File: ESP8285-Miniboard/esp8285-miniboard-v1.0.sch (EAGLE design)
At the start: 40 parts, among them Q1 FA-128

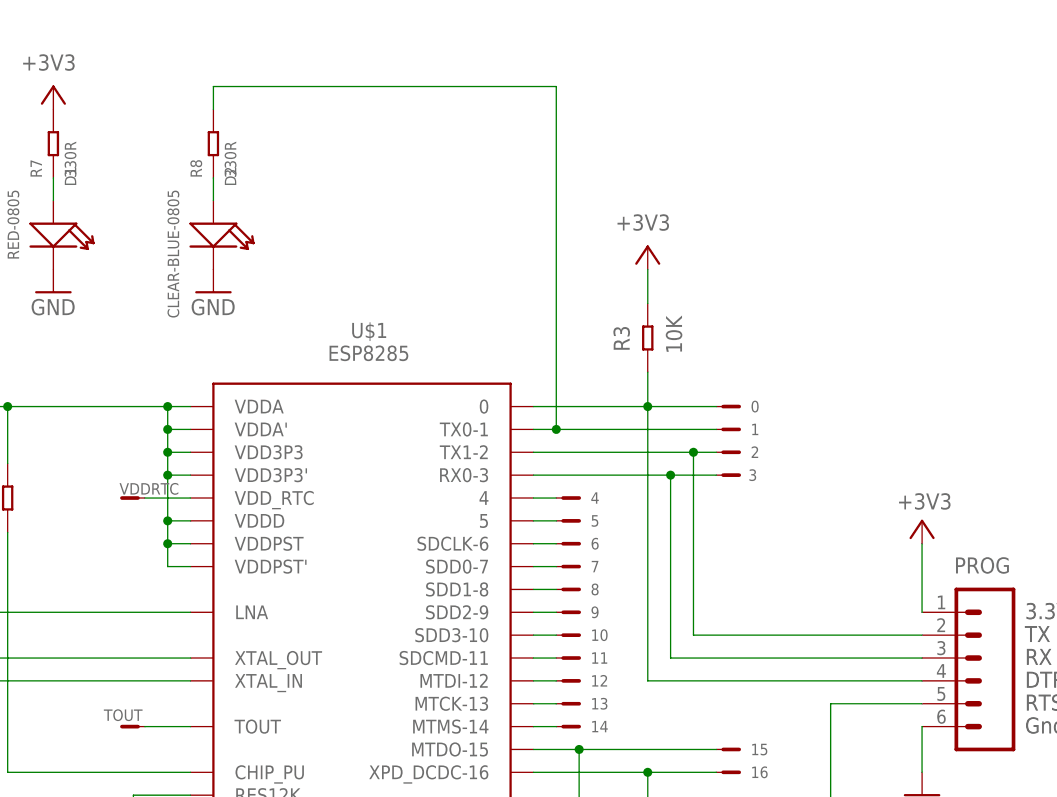
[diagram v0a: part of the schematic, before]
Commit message: Another Rev 1.0
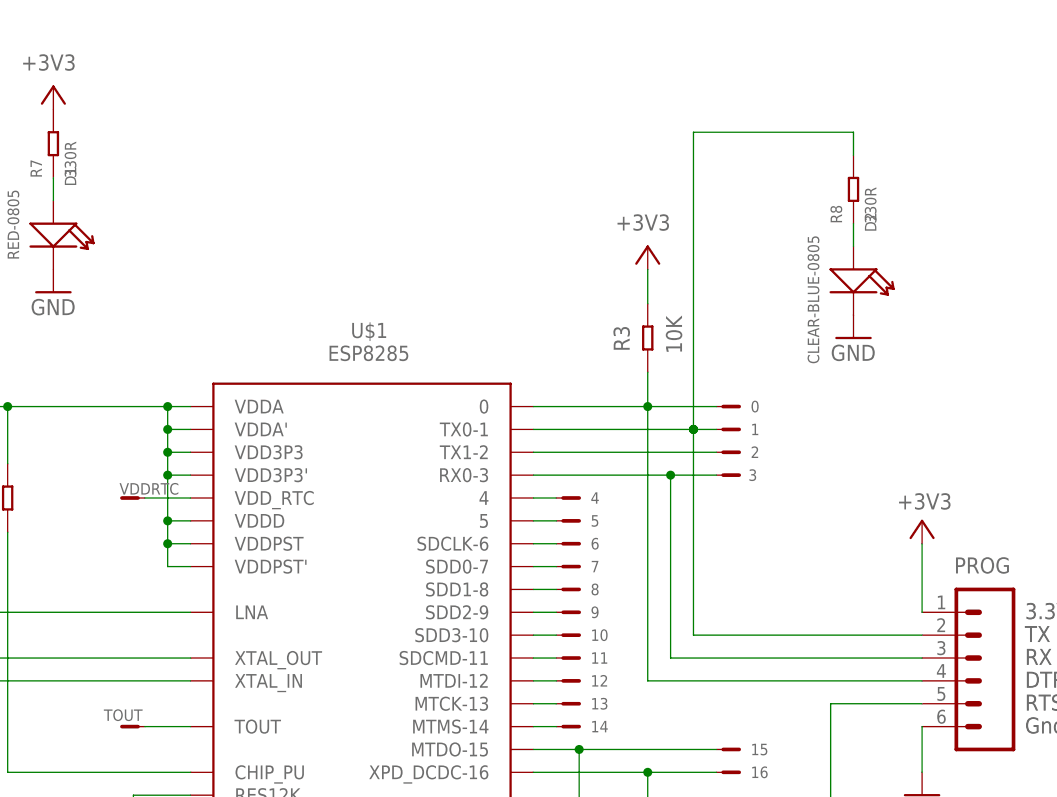
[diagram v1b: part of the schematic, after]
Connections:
- net N$IO1: now also PROG.2
- net N$IO2: no longer PROG.2
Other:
- moved on the sheet: D2, R8
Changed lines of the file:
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@@
 <attribute name="VALUE" x="91.44" y="163.576" size="1.778" layer="96" rot="R180"/>
 </instance>
-<instance part="D2" gate="G$1" x="106.68" y="143.51" rot="R270"/>
-<instance part="R8" gate="G$1" x="106.68" y="153.67" rot="R90"/>
-<instance part="GND13" gate="1" x="106.68" y="137.16"/>
+<instance part="D2" gate="G$1" x="177.8" y="138.43" rot="R270"/>
+<instance part="R8" gate="G$1" x="177.8" y="148.59" rot="R90"/>
+<instance part="GND13" gate="1" x="177.8" y="132.08"/>
 </instances>
 <busses>
@@
 </segment>
 </net>
-<net name="N$IO2" class="0">
-<segment>
-<wire x1="160.02" y1="99.06" x2="185.42" y2="99.06" width="0.1524" layer="91"/>
-<pinref part="PROG" gate="G$1" pin="2"/>
-<pinref part="U$1" gate="G$1" pin="TX1-2"/>
-<pinref part="2" gate="G$1" pin="1"/>
-<wire x1="162.56" y1="119.38" x2="160.02" y2="119.38" width="0.1524" layer="91"/>
-<wire x1="160.02" y1="119.38" x2="142.24" y2="119.38" width="0.1524" layer="91"/>
-<wire x1="160.02" y1="99.06" x2="160.02" y2="119.38" width="0.1524" layer="91"/>
-<junction x="160.02" y="119.38"/>
-</segment>
-</net>
 <net name="N$IO3" class="0">
 <segment>
@@
 <pinref part="D2" gate="G$1" pin="+"/>
 <pinref part="R8" gate="G$1" pin="1"/>
-<wire x1="106.68" y1="149.86" x2="106.68" y2="147.32" width="0.1524" layer="91"/>
+<wire x1="177.8" y1="144.78" x2="177.8" y2="142.24" width="0.1524" layer="91"/>
+</segment>
+</net>
+<net name="N$IO2" class="0">
+<segment>
+<pinref part="U$1" gate="G$1" pin="TX1-2"/>
+<pinref part="2" gate="G$1" pin="1"/>
+<wire x1="162.56" y1="119.38" x2="142.24" y2="119.38" width="0.1524" layer="91"/>
 </segment>
 </net>
 <net name="N$IO1" class="0">
 <segment>
-<wire x1="106.68" y1="160.02" x2="106.68" y2="157.48" width="0.1524" layer="91"/>
+<wire x1="160.02" y1="99.06" x2="185.42" y2="99.06" width="0.1524" layer="91"/>
+<pinref part="PROG" gate="G$1" pin="2"/>
+<wire x1="177.8" y1="154.94" x2="177.8" y2="152.4" width="0.1524" layer="91"/>
 <pinref part="R8" gate="G$1" pin="2"/>
 <pinref part="1" gate="G$1" pin="1"/>
 <pinref part="U$1" gate="G$1" pin="TX0-1"/>
-<wire x1="162.56" y1="121.92" x2="144.78" y2="121.92" width="0.1524" layer="91"/>
-<wire x1="144.78" y1="121.92" x2="142.24" y2="121.92" width="0.1524" layer="91"/>
-<wire x1="106.68" y1="160.02" x2="144.78" y2="160.02" width="0.1524" layer="91"/>
-<wire x1="144.78" y1="160.02" x2="144.78" y2="121.92" width="0.1524" layer="91"/>
-<junction x="144.78" y="121.92"/>
-</segment>
-</net>
+<wire x1="162.56" y1="121.92" x2="160.02" y2="121.92" width="0.1524" layer="91"/>
+<wire x1="160.02" y1="121.92" x2="142.24" y2="121.92" width="0.1524" layer="91"/>
+<wire x1="177.8" y1="154.94" x2="160.02" y2="154.94" width="0.1524" layer="91"/>
+<wire x1="160.02" y1="154.94" x2="160.02" y2="121.92" width="0.1524" layer="91"/>
+<junction x="160.02" y="121.92"/>
+<wire x1="160.02" y1="99.06" x2="160.02" y2="121.92" width="0.1524" layer="91"/>
+<junction x="160.02" y="121.92"/>
+</segment>
+</net>
